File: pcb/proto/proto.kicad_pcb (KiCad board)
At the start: 2 copper layers, 50.8 x 25.4 mm, 12 parts, among them U1 AMS1117-3.3, U2 CH340C, U3 F030F4Px

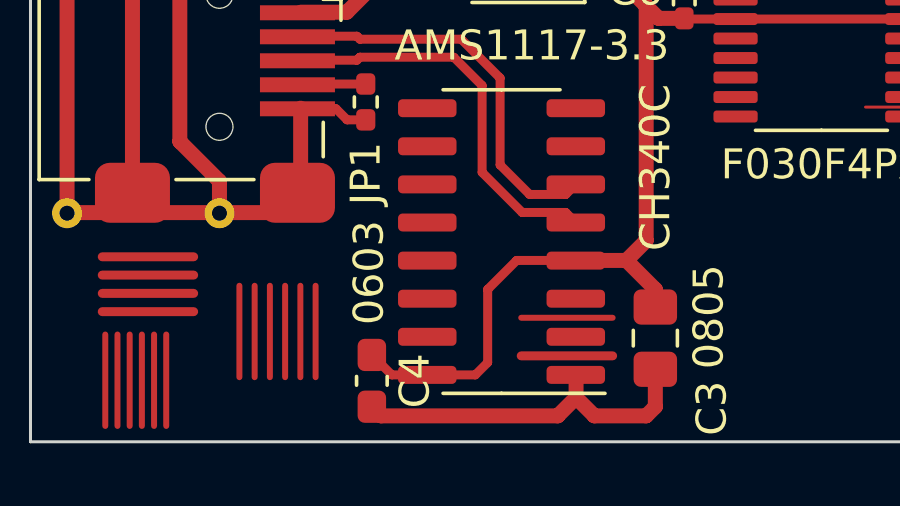
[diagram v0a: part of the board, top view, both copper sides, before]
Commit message: Signed-off-by: Dmitry Ponyatov <ponyatov@example.com>
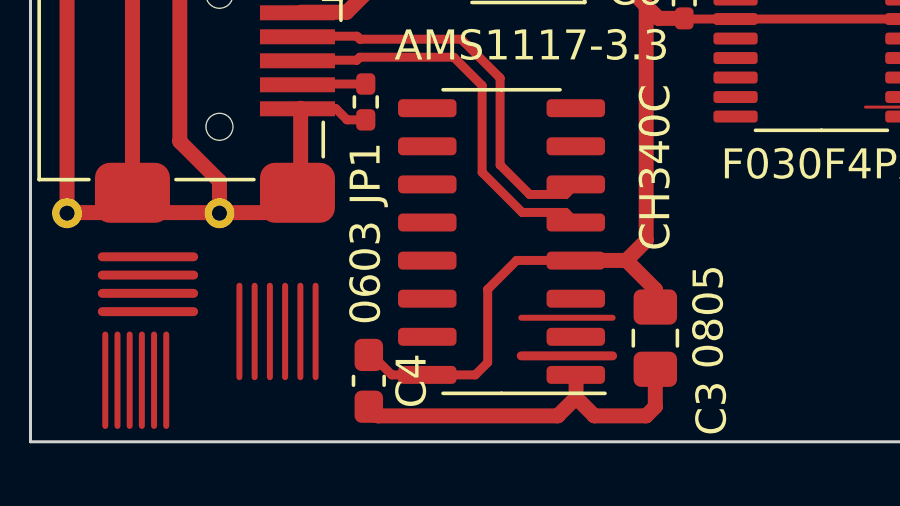
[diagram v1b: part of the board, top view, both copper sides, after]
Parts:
- moved C4 0.10 mm to (112.9, 99.6)
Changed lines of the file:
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@@
   )
   (footprint "Capacitor_SMD:C_0603_1608Metric_Pad1.08x0.95mm_HandSolder" (layer "F.Cu")
-    (at 112.9792 99.568 -90)
+    (at 112.8776 99.568 -90)
     (descr "Capacitor SMD 0603 (1608 Metric), square (rectangular) end terminal, IPC_7351 nominal with elongated pad for handsoldering. (Body size source: IPC-SM-782 page 76, https://www.pcb-3d.com/wordpress/wp-content/uploads/ipc-sm-782a_amendment_1_and_2.pdf), generated with kicad-footprint-generator")
     (tags "capacitor handsolder")
@@
   (segment (start 108.0052 93.9604) (end 109.9252 93.9604) (width 0.5) (layer "F.Cu") (net 31))
   (segment (start 124.4854 77.3938) (end 122.2502 77.3938) (width 0.5) (layer "F.Cu") (net 31))
+  (segment (start 119.7864 100.1268) (end 119.1768 100.7364) (width 0.5) (layer "F.Cu") (net 31))
   (segment (start 102.9252 93.9604) (end 104.4252 93.9604) (width 0.5) (layer "F.Cu") (net 31))
   (segment (start 104.4252 93.9604) (end 105.1052 93.2804) (width 0.5) (layer "F.Cu") (net 31))
@@
   (segment (start 133.4472 87.6496) (end 132.736 88.3608) (width 0.5) (layer "F.Cu") (net 31))
   (segment (start 104.4252 83.8004) (end 105.1052 84.4804) (width 0.5) (layer "F.Cu") (net 31))
-  (segment (start 119.7864 100.1268) (end 119.1768 100.7364) (width 0.5) (layer "F.Cu") (net 31))
-  (segment (start 119.1768 100.7364) (end 113.2851 100.7364) (width 0.5) (layer "F.Cu") (net 31))
   (segment (start 131.884717 88.3499) (end 131.693017 88.1582) (width 0.3) (layer "F.Cu") (net 31))
   (segment (start 114.3552 79.3554) (end 114.9902 79.9904) (width 0.5) (layer "F.Cu") (net 31))
@@
   (segment (start 118.1579 77.4192) (end 116.6027 78.9744) (width 0.5) (layer "F.Cu") (net 31))
   (segment (start 108.9302 81.2604) (end 108.9302 80.0814) (width 0.5) (layer "F.Cu") (net 31))
+  (segment (start 113.1835 100.7364) (end 112.8776 100.4305) (width 0.5) (layer "F.Cu") (net 31))
   (segment (start 106.5784 86.3092) (end 107.8992 84.9884) (width 0.5) (layer "F.Cu") (net 31))
   (segment (start 133.4472 85.0856) (end 133.4472 87.6496) (width 0.5) (layer "F.Cu") (net 31))
@@
   (segment (start 108.0052 93.9604) (end 105.7852 93.9604) (width 0.5) (layer "F.Cu") (net 31))
   (segment (start 120.396 100.7364) (end 119.7864 100.1268) (width 0.5) (layer "F.Cu") (net 31))
-  (segment (start 113.2851 100.7364) (end 112.9792 100.4305) (width 0.5) (layer "F.Cu") (net 31))
   (segment (start 105.7852 83.8004) (end 105.1052 84.4804) (width 0.5) (layer "F.Cu") (net 31))
   (segment (start 111.7852 90.5) (end 110.4992 90.5) (width 0.3) (layer "F.Cu") (net 31))
@@
   (segment (start 111.104 96.3988) (end 111.104 99.4468) (width 0.2) (layer "F.Cu") (net 31))
   (segment (start 104.9992 93.3) (end 104.9992 84.5) (width 0.5) (layer "F.Cu") (net 31))
+  (segment (start 119.1768 100.7364) (end 113.1835 100.7364) (width 0.5) (layer "F.Cu") (net 31))
   (segment (start 123.3932 84.3788) (end 123.3932 86.3513) (width 0.5) (layer "F.Cu") (net 31))
   (segment (start 124.7648 82.7024) (end 122.1232 80.0608) (width 0.5) (layer "F.Cu") (net 31))
